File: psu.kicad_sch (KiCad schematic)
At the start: 38 parts, among them J6 Screw_Terminal_01x02, J7 Barrel_Jack_MountingPin, Q1 FDS4435BZ, U13 LT3045EMSE#PBF, U15 TPS7A2033PDBVR, U5 TPS7A2033PDBVR, U6 TPS56637RPAR

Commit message: a few edits
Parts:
- U6: footprint Pedalboard Library:RPA0010A -> RPA0010A
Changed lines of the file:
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@@
 			)
 		)
-		(property "Footprint" "Pedalboard Library:RPA0010A"
+		(property "Footprint" "RPA0010A"
 			(at 119.38 130.81 0)
 			(hide yes)

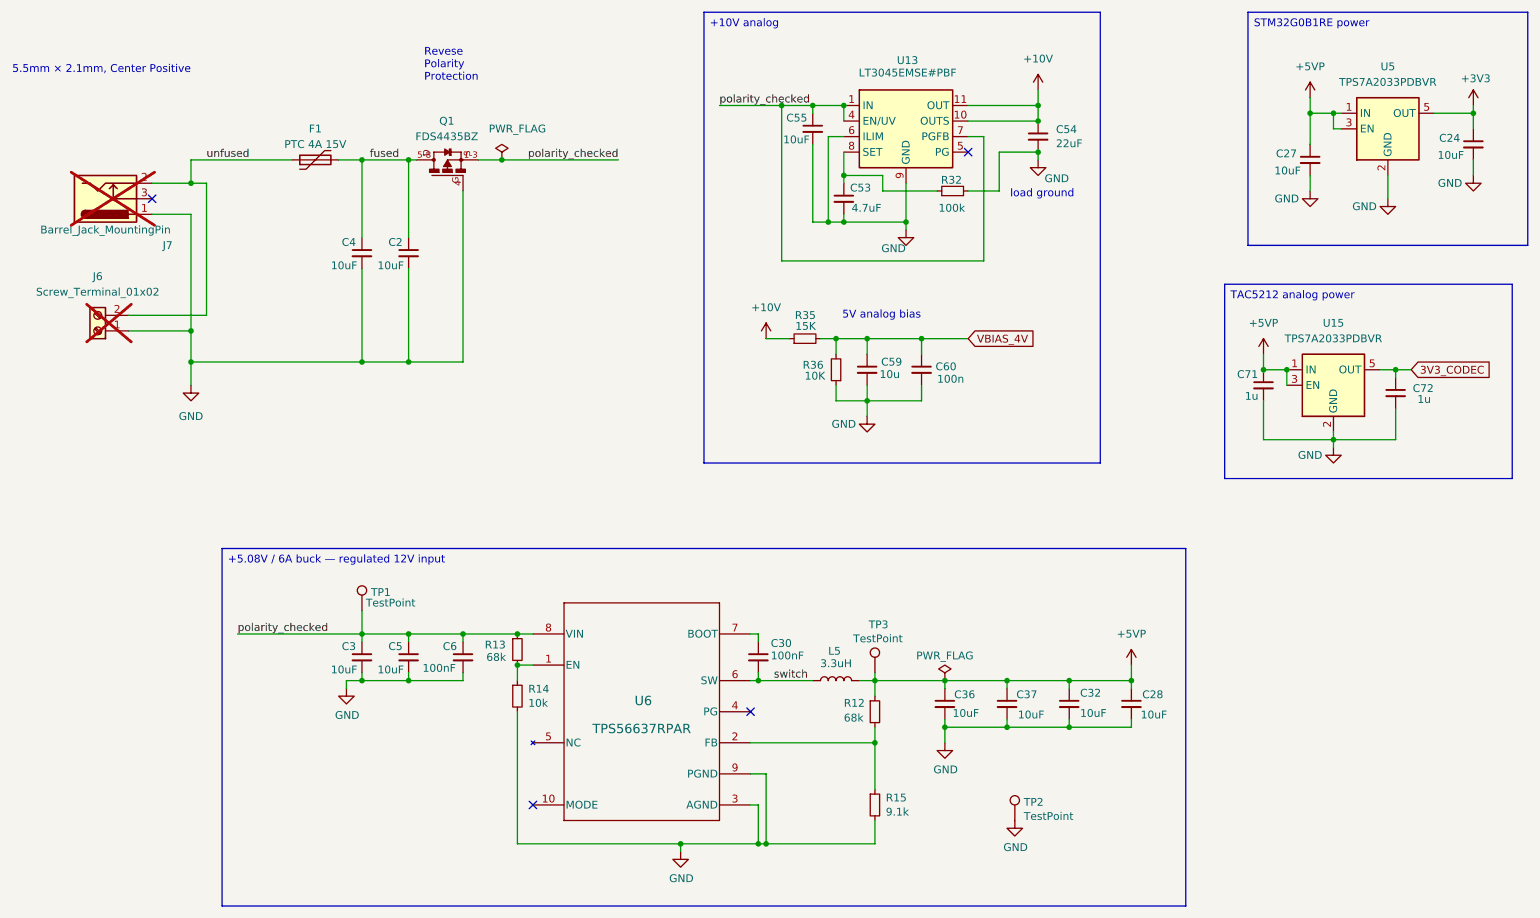
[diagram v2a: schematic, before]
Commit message: fixed warnings.
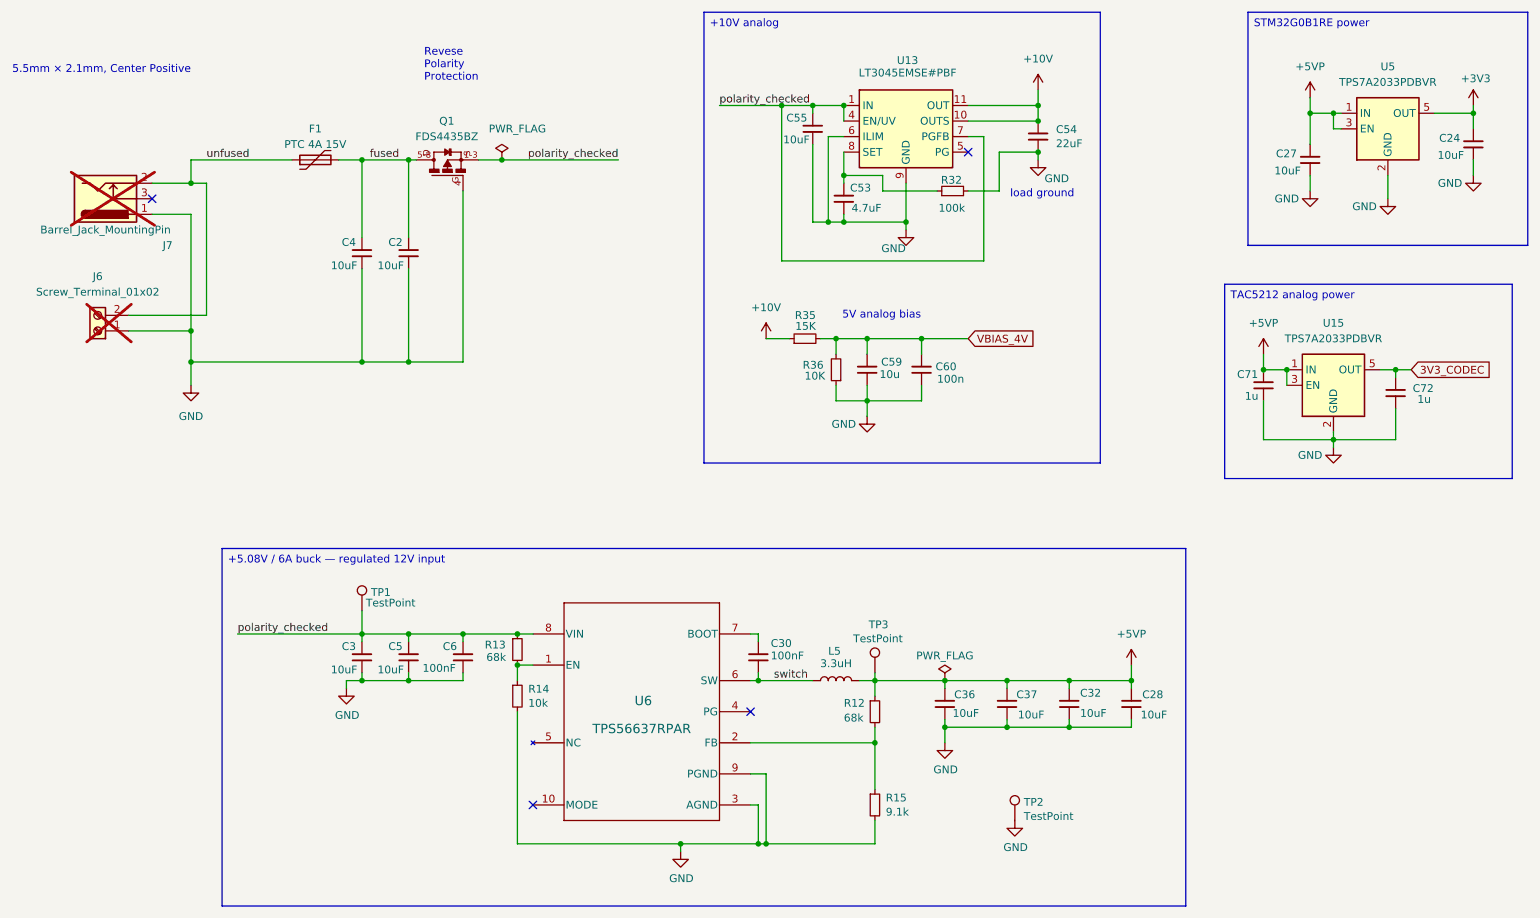
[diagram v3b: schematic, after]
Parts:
- U6: footprint RPA0010A -> Pedalboard Library:RPA0010A
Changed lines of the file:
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@@
 			)
 		)
-		(property "Footprint" "RPA0010A"
+		(property "Footprint" "Pedalboard Library:RPA0010A"
 			(at 119.38 130.81 0)
 			(hide yes)
